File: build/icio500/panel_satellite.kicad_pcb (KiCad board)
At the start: 2 copper layers, 38.1 x 133.3 mm, 32 parts, among them J1 Conn_02x10_Odd_Even, U1 IS31FL3236

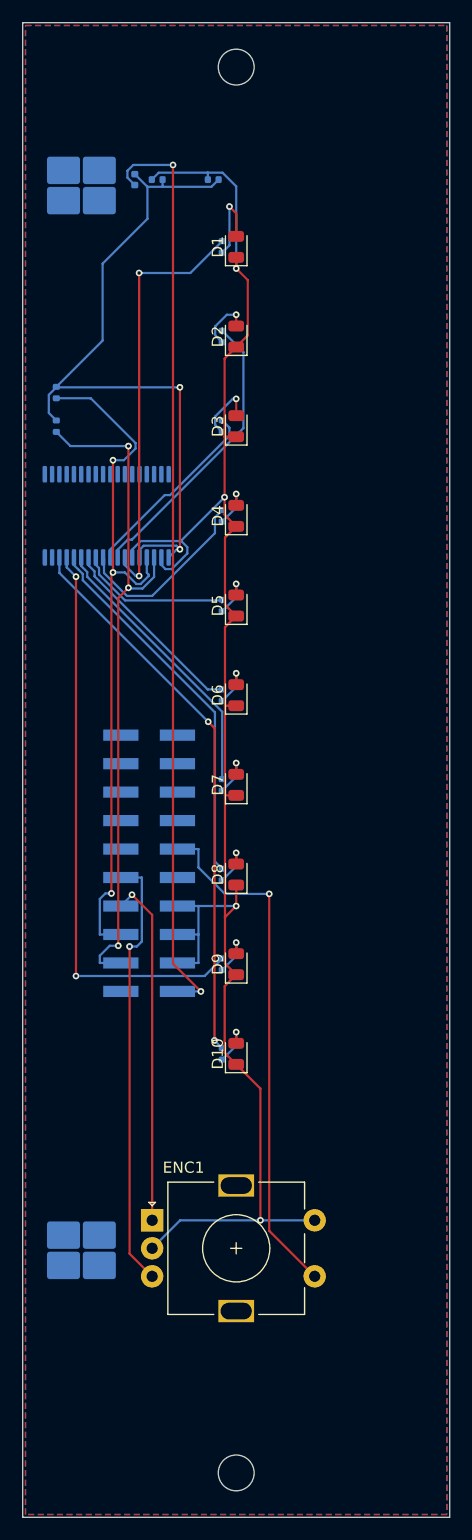
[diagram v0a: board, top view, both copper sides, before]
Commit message: Restore finished 10-27 faceplate & satellite; maintain summer VPR card edge with zero DRC violations
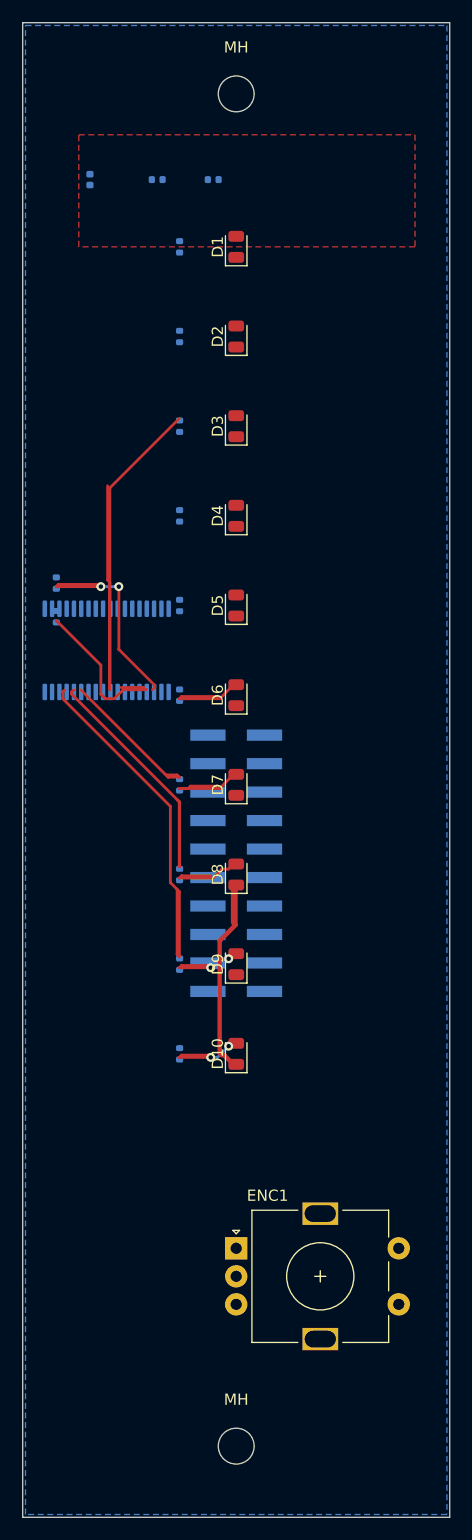
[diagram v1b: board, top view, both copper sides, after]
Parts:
- removed BR1, BR2: WP-SMRA-M3, Mounting_Wuerth_WP-SMRA-M3_L7mm_7466303_Horizontal
- moved R12 20.0 mm to (103.0, 153.0)
- moved R11 14.0 mm to (103.0, 150.0)
- moved U1 12.0 mm to (107.5, 156.0)
- moved ENC1 7.91 mm to (119.0, 209.3)
- moved J1 7.77 mm to (119.0, 175.0)
- moved FB1 4.00 mm to (106.0, 114.0)
- moved R1 3.80 mm to (114.0, 120.0)
- moved R10 3.80 mm to (114.0, 192.0)
- moved R2 3.80 mm to (114.0, 128.0)
- moved R3 3.80 mm to (114.0, 136.0)
- moved R4 3.80 mm to (114.0, 144.0)
- moved R5 3.80 mm to (114.0, 152.0)
- moved R6 3.80 mm to (114.0, 160.0)
- moved R7 3.80 mm to (114.0, 168.0)
- moved R8 3.80 mm to (114.0, 176.0)
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- renumbered MH1 to MH, MH2 to MH
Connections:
- C1 pad 1: +3V3 -> (no net)
- C1 pad 2: GND -> (no net)
- C2 pad 1: +3V3 -> (no net)
- C2 pad 2: GND -> (no net)
- D1 pad 1: GND -> (no net)
- D1 pad 2: LED_1_MID -> (no net)
- D2 pad 1: GND -> (no net)
- D2 pad 2: LED_2_MID -> (no net)
- D3 pad 1: GND -> (no net)
- D3 pad 2: LED_3_MID -> (no net)
- D4 pad 1: GND -> (no net)
- D4 pad 2: LED_4_MID -> (no net)
- D5 pad 1: GND -> (no net)
- D5 pad 2: LED_5_MID -> (no net)
- D6 pad 1: GND -> (no net)
- D7 pad 1: GND -> (no net)
- D9 pad 1: GND -> (no net)
- ENC1 pad A: ENC_A -> (no net)
- ENC1 pad B: ENC_B -> (no net)
- ENC1 pad C: GND -> (no net)
- ENC1 pad S1: ENC_SW -> (no net)
- ENC1 pad S2: GND -> (no net)
- FB1 pad 1: +3V3_IN -> (no net)
- FB1 pad 2: +3V3 -> (no net)
- J1 pad 12: ENC_SW -> (no net)
- J1 pad 2: +3V3_IN -> (no net)
- J1 pad 3: SDA -> (no net)
- J1 pad 4: GND -> (no net)
- J1 pad 5: SCL -> (no net)
- J1 pad 6: GND -> (no net)
- J1 pad 7: ENC_A -> (no net)
- J1 pad 8: GND -> (no net)
- J1 pad 9: ENC_B -> (no net)
- R1 pad 1: LED_1_MID -> (no net)
- R1 pad 2: LED_1 -> (no net)
- R11 pad 2: +3V3 -> (no net)
- R12 pad 2: +3V3 -> (no net)
- R4 pad 1: LED_4_MID -> (no net)
- R4 pad 2: LED_4 -> (no net)
- R5 pad 1: LED_5_MID -> (no net)
- R5 pad 2: LED_5 -> (no net)
- R6 pad 2: LED_6 -> (no net)
- U1 pad 1: +3V3 -> (no net)
- U1 pad 16: LED_10 -> (no net)
- U1 pad 2: GND -> (no net)
- U1 pad 5: +3V3 -> (no net)
- U1 pad 6: GND -> (no net)
- U1 pad 7: LED_1 -> (no net)
- U1 pad 8: LED_2 -> (no net)
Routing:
- net GND: track 159.2 -> 20.9 mm, vias 4 -> 0
- net +3V3_IN: track 82.7 -> 0.00 mm, vias 2 -> 0
- net +3V3: track 65.0 -> 0.00 mm, vias 2 -> 0
- net LED_10: track 49.8 -> 0.00 mm, vias 2 -> 0
- net SCL: track 62.3 -> 15.0 mm, vias 3 -> 0
- net ENC_SW: track 46.6 -> 0.00 mm, vias 1 -> 0
- net SDA: track 60.9 -> 20.1 mm, vias 3 -> 0
- net ENC_B: track 39.1 -> 0.00 mm, vias 1 -> 0
- net LED_1: track 38.0 -> 0.00 mm, vias 2 -> 0
- net ENC_A: track 31.2 -> 0.00 mm, vias 1 -> 0
- net LED_3: track 17.2 -> 45.1 mm
- net LED_2: track 25.9 -> 0.00 mm
- net LED_6: track 17.5 -> 0.00 mm
- net LED_9: track 51.4 -> 34.3 mm, vias 2 -> 0
- net LED_4: track 16.8 -> 0.00 mm
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- added copper zone on B.Cu, net (none)
- added copper zone on F.Cu, net (none)
- removed copper zone on B.Cu, net GND
- removed copper zone on F.Cu, net GND
